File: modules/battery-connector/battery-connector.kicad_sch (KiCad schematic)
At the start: 2 parts, among them J1 691210910002

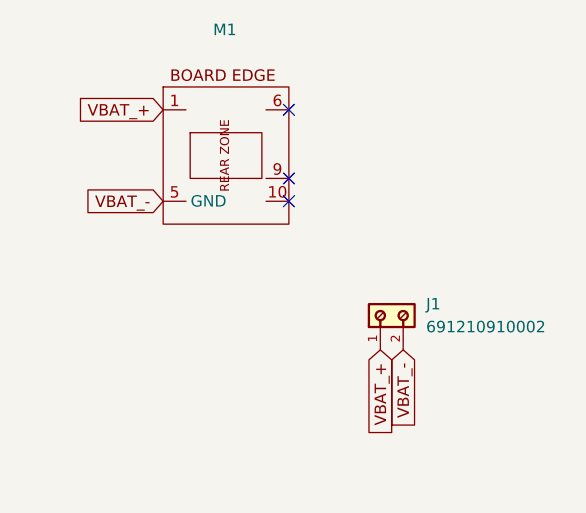
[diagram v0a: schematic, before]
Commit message: Update one board - checking workflow
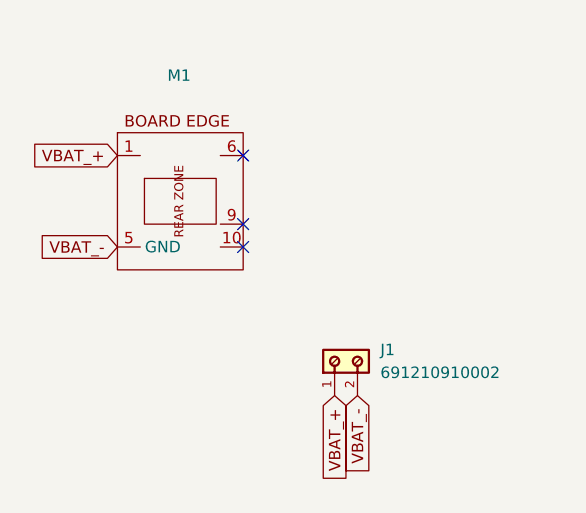
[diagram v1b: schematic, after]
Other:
- moved on the sheet: J1, M1
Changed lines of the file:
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@@
 	(paper "A4")
 	(no_connect
-		(at 113.03 41.91)
+		(at 107.95 46.99)
 	)
 	(no_connect
-		(at 113.03 34.29)
+		(at 107.95 39.37)
 	)
 	(no_connect
-		(at 113.03 44.45)
+		(at 107.95 49.53)
 	)
 	(global_label "VBAT_+"
 		(shape input)
-		(at 99.06 34.29 180)
+		(at 93.98 39.37 180)
 		(fields_autoplaced yes)
 		(effects
@@
 		)
 		(property "Intersheetrefs" "${INTERSHEET_REFS}"
-			(at 89.12 34.29 0)
+			(at 84.04 39.37 0)
 			(effects
 				(font
@@
 	(global_label "VBAT_-"
 		(shape input)
-		(at 99.06 44.45 180)
+		(at 93.98 49.53 180)
 		(fields_autoplaced yes)
 		(effects
@@
 		)
 		(property "Intersheetrefs" "${INTERSHEET_REFS}"
-			(at 89.12 44.45 0)
+			(at 84.04 49.53 0)
 			(effects
 				(font
@@
 	(global_label "VBAT_-"
 		(shape input)
-		(at 125.73 60.96 270)
+		(at 120.65 66.04 270)
 		(fields_autoplaced yes)
 		(effects
@@
 		)
 		(property "Intersheetrefs" "${INTERSHEET_REFS}"
-			(at 125.73 70.9 90)
+			(at 120.65 75.98 90)
 			(effects
 				(font
@@
 	(global_label "VBAT_+"
 		(shape input)
-		(at 123.19 60.96 270)
+		(at 118.11 66.04 270)
 		(fields_autoplaced yes)
 		(effects
@@
 		)
 		(property "Intersheetrefs" "${INTERSHEET_REFS}"
-			(at 123.19 70.9 90)
+			(at 118.11 75.98 90)
 			(effects
 				(font
@@
 	(symbol
 		(lib_id "MegaCastle:MegaCastle2x5-Module-I7.0x7.9-M8CC-EDGE")
-		(at 105.41 39.37 0)
+		(at 100.33 44.45 0)
 		(unit 1)
 		(exclude_from_sim no)
@@
 		(fields_autoplaced yes)
 		(property "Reference" "M1"
-			(at 105.9138 25.4 0)
+			(at 100.8338 30.48 0)
 			(effects
 				(font
@@
 		)
 		(property "Value" "~"
-			(at 105.9138 27.94 0)
+			(at 100.8338 33.02 0)
 			(effects
 				(font
@@
 		)
 		(property "Footprint" "MegaCastle:MegaCastle2x5-Module-I15.0x7.9-M8CC-SPAREPAD"
-			(at 105.41 52.07 0)
+			(at 100.33 57.15 0)
 			(effects
 				(font
@@
 		)
 		(property "Datasheet" ""
-			(at 105.41 34.29 0)
+			(at 100.33 39.37 0)
 			(effects
 				(font
@@
 		)
 		(property "Description" "Generated using footprint-gen .. 7 8 5 M8CC"
-			(at 105.41 39.37 0)
+			(at 100.33 44.45 0)
 			(effects
 				(font
@@
 	(symbol
 		(lib_id "691210910002:691210910002")
-		(at 125.73 55.88 0)
+		(at 120.65 60.96 0)
 		(unit 1)
 		(exclude_from_sim no)
@@
 		(fields_autoplaced yes)
 		(property "Reference" "J1"
-			(at 128.27 55.8799 0)
+			(at 123.19 60.9599 0)
 			(effects
 				(font
@@
 		)
 		(property "Value" "691210910002"
-			(at 128.27 58.4199 0)
+			(at 123.19 63.4999 0)
 			(effects
 				(font
@@
 		)
 		(property "Footprint" "MegaCastle:691210910002"
-			(at 125.73 55.88 0)
+			(at 120.65 60.96 0)
 			(effects
 				(font
@@
 		)
 		(property "Datasheet" ""
-			(at 125.73 55.88 0)
+			(at 120.65 60.96 0)
 			(effects
 				(font
@@
 		)
 		(property "Description" ""
-			(at 125.73 55.88 0)
+			(at 120.65 60.96 0)
 			(effects
 				(font
@@
 		)
 		(property "WIRE" "30 to 18 (AWG) 0.0509 to 0.823 (mm²)"
-			(at 125.73 55.88 0)
+			(at 120.65 60.96 0)
 			(effects
 				(font
@@
 		)
 		(property "MOUNT" "THT"
-			(at 125.73 55.88 0)
+			(at 120.65 60.96 0)
 			(effects
 				(font
@@
 		)
 		(property "IR-UL" "6A"
-			(at 125.73 55.88 0)
+			(at 120.65 60.96 0)
 			(effects
 				(font
@@
 		)
 		(property "WORKING-VOLTAGE-UL" "150V (AC)"
-			(at 125.73 55.88 0)
+			(at 120.65 60.96 0)
 			(effects
 				(font
@@
 		)
 		(property "PART-NUMBER" "691210910002"
-			(at 125.73 55.88 0)
+			(at 120.65 60.96 0)
 			(effects
 				(font
@@
 		)
 		(property "DATASHEET-URL" "https://www.we-online.com/redexpert/spec/691210910002?ae"
-			(at 125.73 55.88 0)
+			(at 120.65 60.96 0)
 			(effects
 				(font
@@
 		)
 		(property "PITCH" "2.54mm"
-			(at 125.73 55.88 0)
+			(at 120.65 60.96 0)
 			(effects
 				(font
@@
 		)
 		(property "PINS" "2"
-			(at 125.73 55.88 0)
+			(at 120.65 60.96 0)
 			(effects
 				(font
@@
 		)
 		(property "TYPE" "Horizontal"
-			(at 125.73 55.88 0)
-			(effects
-				(font
+			(at 120.65 60.96 0)
+			(effects
+				(font
